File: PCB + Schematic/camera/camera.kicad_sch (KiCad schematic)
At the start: 26 parts, among them J1 Micro_SD_Card, J2 Camera, Q1 PMOS, SW1 RESET, U1 ESP32-S3-WROOM-1, U2 AMS1117-3.3, U3 XC6206-2.8, U4 XC6206-1.2

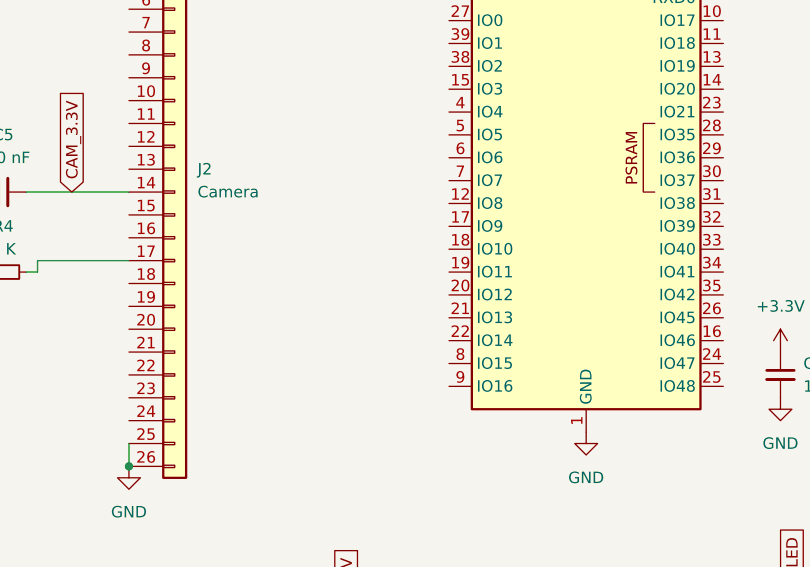
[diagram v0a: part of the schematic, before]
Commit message: Commit
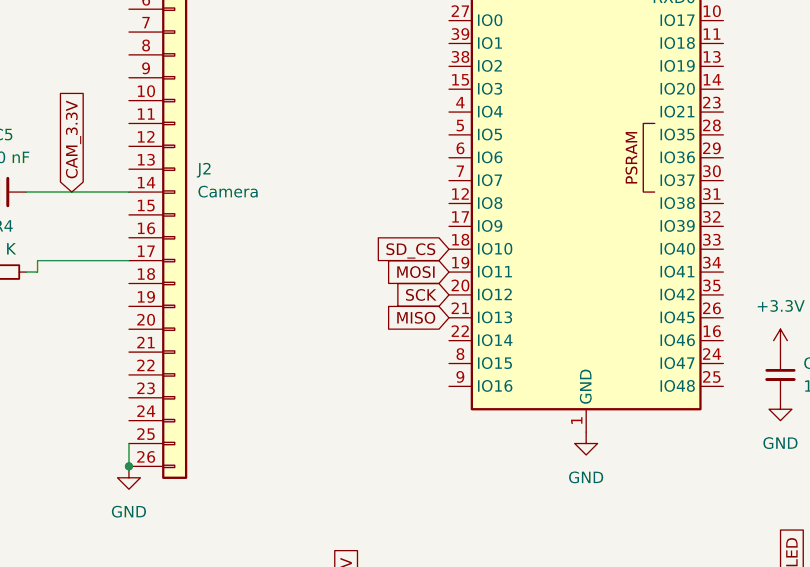
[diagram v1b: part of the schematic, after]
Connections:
- net MISO: now also U1.21 (IO13)
- net MOSI: now also U1.19 (IO11)
- net SCK: now also U1.20 (IO12)
- net SD_CS: now also U1.18 (IO10)
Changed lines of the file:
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@@
+		)
+	)
+	(global_label "MISO"
+		(shape input)
+		(at 142.24 100.33 180)
+		(fields_autoplaced yes)
+		(effects
+			(font
+				(size 1.27 1.27)
+			)
+			(justify right)
+		)
+		(property "Intersheetrefs" "${INTERSHEET_REFS}"
+			(at 134.6586 100.33 0)
+			(effects
+				(font
+					(size 1.27 1.27)
+				)
+				(justify right)
+				(hide yes)
+			)
 		)
 	)
@@
 		)
 	)
+	(global_label "SD_CS"
+		(shape input)
+		(at 142.24 92.71 180)
+		(fields_autoplaced yes)
+		(effects
+			(font
+				(size 1.27 1.27)
+			)
+			(justify right)
+		)
+		(property "Intersheetrefs" "${INTERSHEET_REFS}"
+			(at 133.3282 92.71 0)
+			(effects
+				(font
+					(size 1.27 1.27)
+				)
+				(justify right)
+				(hide yes)
+			)
+		)
+	)
 	(global_label "MOSI"
 		(shape input)
@@
 		)
 	)
+	(global_label "SCK"
+		(shape input)
+		(at 142.24 97.79 180)
+		(fields_autoplaced yes)
+		(effects
+			(font
+				(size 1.27 1.27)
+			)
+			(justify right)
+		)
+		(property "Intersheetrefs" "${INTERSHEET_REFS}"
+			(at 135.5053 97.79 0)
+			(effects
+				(font
+					(size 1.27 1.27)
+				)
+				(justify right)
+				(hide yes)
+			)
+		)
+	)
 	(global_label "SD_CS"
 		(shape input)
@@
 			(effects
 				(font
+					(size 1.27 1.27)
+				)
+				(justify right)
+				(hide yes)
+			)
+		)
+	)
+	(global_label "MOSI"
+		(shape input)
+		(at 142.24 95.25 180)
+		(fields_autoplaced yes)
+		(effects
+			(font
+				(size 1.27 1.27)
+			)
+			(justify right)
+		)
+		(property "Intersheetrefs" "${INTERSHEET_REFS}"
+			(at 134.6586 95.25 0)
+			(effects
+				(font
